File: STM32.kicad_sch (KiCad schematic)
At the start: 16 parts, among them IC1 TCAN3413DRBR, SW3 SW_SPDT, SW4 SW_Push, U1 STM32F072RBH6

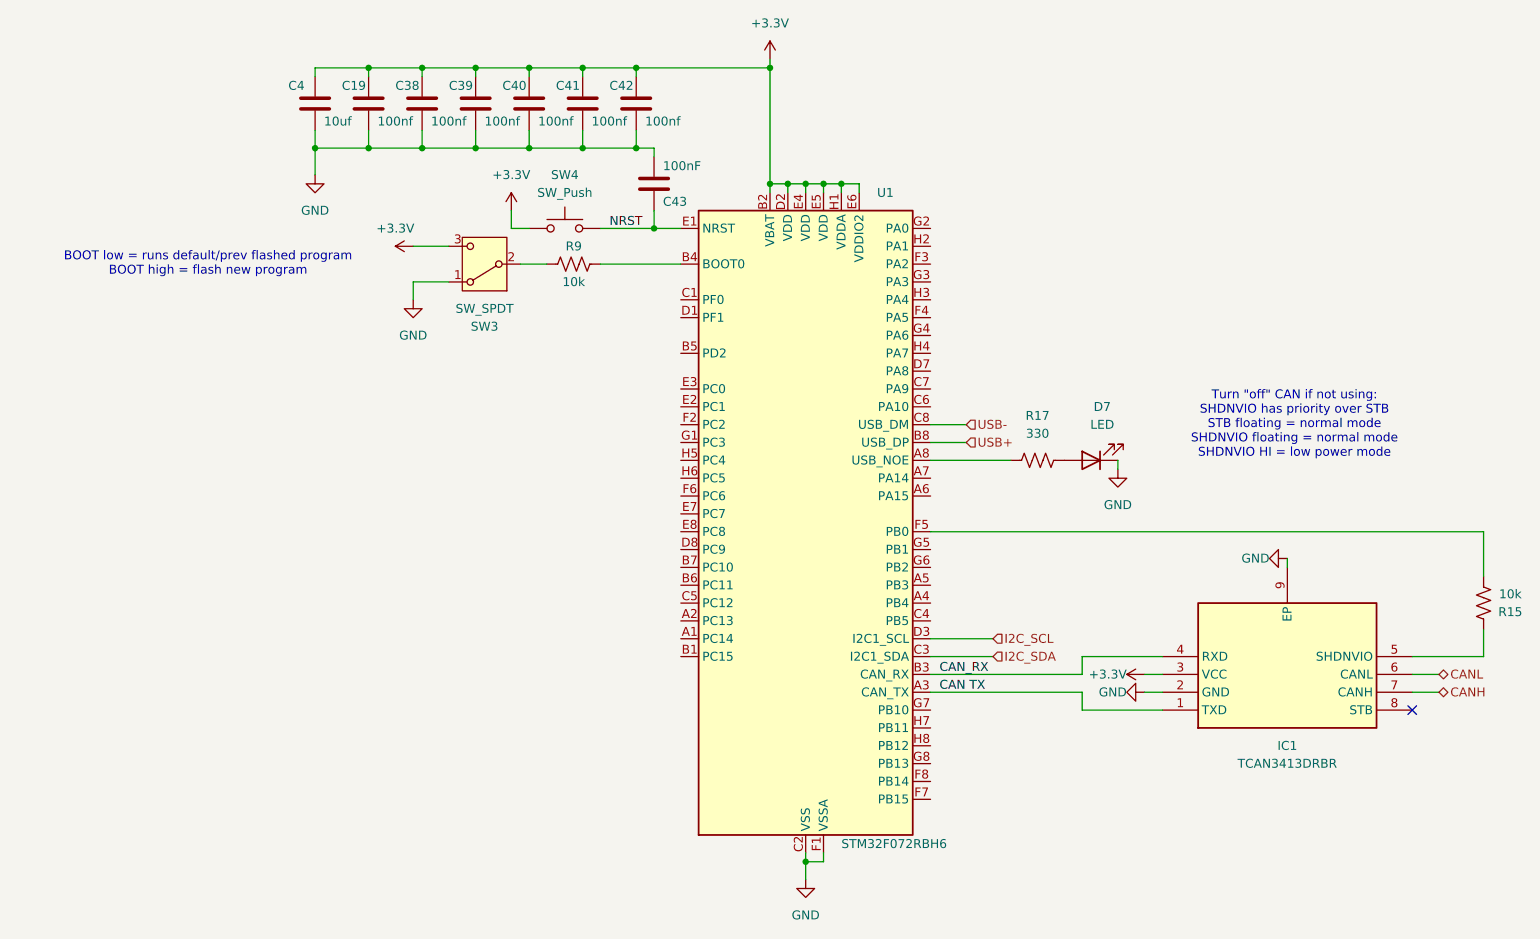
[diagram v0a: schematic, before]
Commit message: routed stm32
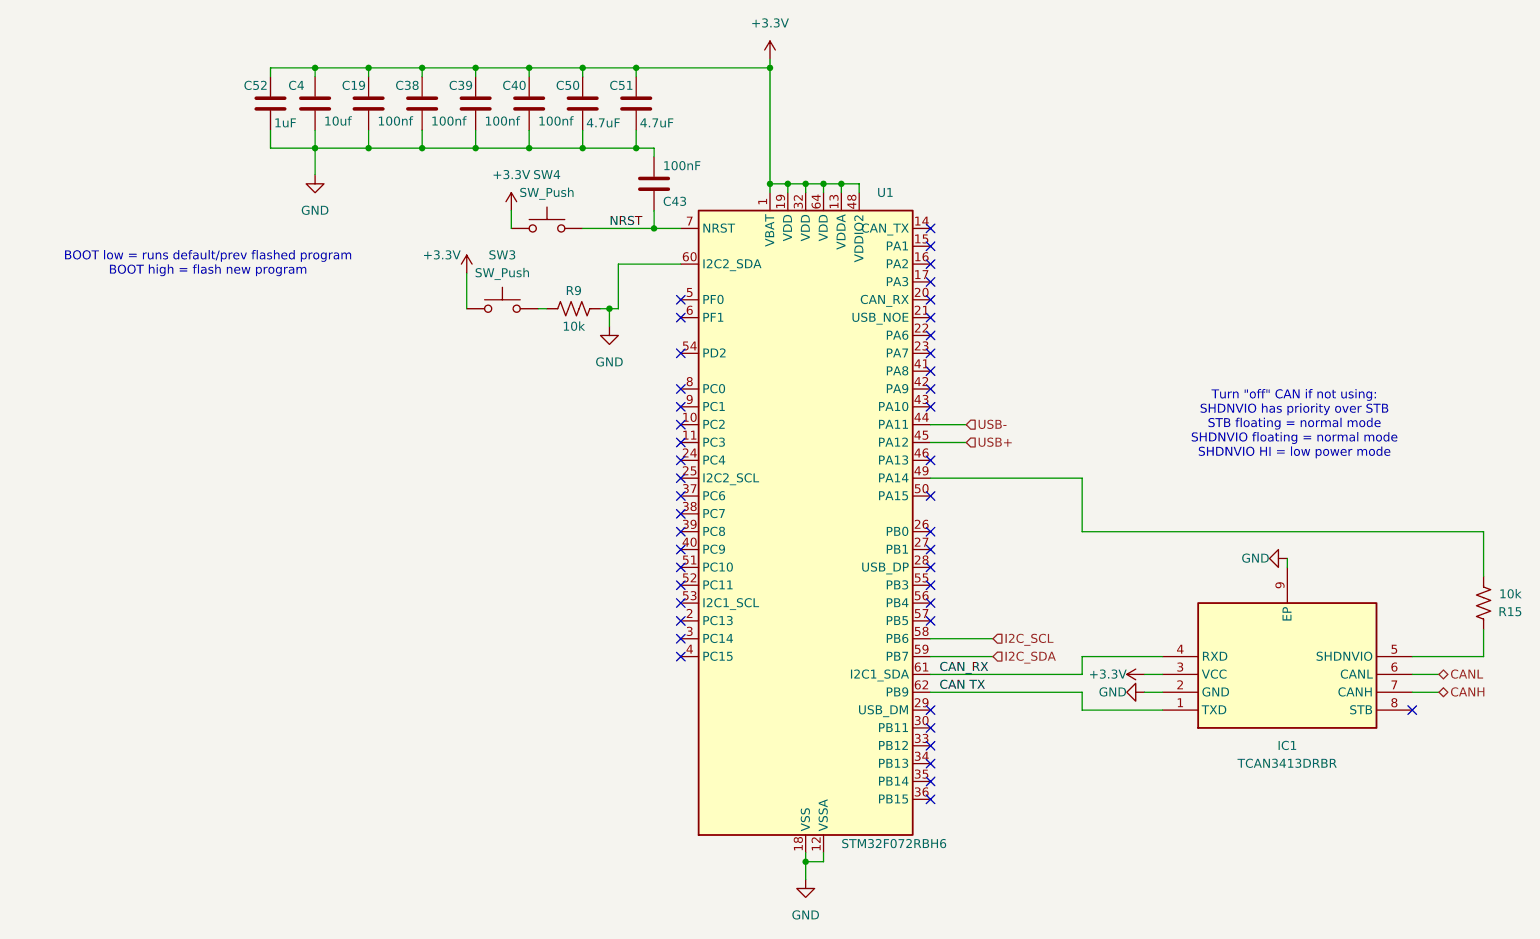
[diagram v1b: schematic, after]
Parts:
- removed C41, C42: 100nf, Capacitor_SMD:C_0603_1608Metric, symbol Device:C
- removed D7: LED, LED_SMD:LED_0603_1608Metric, symbol Device:LED
- removed R17: 330, Resistor_SMD:R_0603_1608Metric, symbol Device:R_US
- removed SW3: SW_SPDT, Button_Switch_SMD:SW_SPDT_PCM12, symbol Switch:SW_SPDT
- added C50, C51: 4.7uF, Capacitor_SMD:C_0603_1608Metric, symbol Device:C
- added C52: 1uF, Capacitor_SMD:C_0603_1608Metric, symbol Device:C
- added SW3: SW_Push, Button_Switch_SMD:SW_Push_1P1T_XKB_TS-1187A, symbol Switch:SW_Push
- U1: footprint Package_BGA:UFBGA-64_5x5mm_Layout8x8_P0.5mm -> Package_QFP:LQFP-64_10x10mm_P0.5mm; symbol MCU_ST_STM32F0:STM32F072RBHx -> MCU_ST_STM32F0:STM32F072RBTx
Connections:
- net +3.3V: now also U1.1 (VBAT), U1.13 (VDDA), U1.19 (VDD), U1.32 (VDD), U1.48 (VDDIO2), U1.64 (VDD), C50.1, C51.1, C52.1, SW3.1; no longer U1.B2 (VBAT), U1.D2 (VDD), U1.E4 (VDD), U1.E5 (VDD), U1.E6 (VDDIO2), U1.H1 (VDDA)
- net CAN TX: now also U1.62 (PB9); no longer U1.A3 (PB9)
- net CAN_RX: now also U1.61 (PB8); no longer U1.B3 (PB8)
- net GND: now also R9.2, U1.12 (VSSA), U1.18 (VSS), U1.31 (VSS), U1.47 (VSS), U1.60 (BOOT0), U1.63 (VSS), C50.2, C51.2, C52.2; no longer U1.C2 (VSS), U1.D4 (VSS), U1.D5 (VSS), U1.D6 (VSS), U1.F1 (VSSA)
- net I2C_SCL: now also U1.58 (PB6); no longer U1.D3 (PB6)
- net I2C_SDA: now also U1.59 (PB7); no longer U1.C3 (PB7)
- net NRST: now also U1.7 (NRST); no longer U1.E1 (NRST)
- net USB+: now also U1.45 (PA12); no longer U1.B8 (PA12)
- net USB-: now also U1.44 (PA11); no longer U1.C8 (PA11)
- net at R15.1: now also U1.49 (PA14); no longer U1.F5 (PB0)
- net at R9.1: now also SW3.2
- no-connect marks 1 -> 45
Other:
- moved on the sheet: R9, SW4
